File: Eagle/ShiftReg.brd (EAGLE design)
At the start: 100 x 80 mm, 206 parts, among them Q10 310mA/60V/1.6Ω, Q100 310mA/60V/1.6Ω, Q101 310mA/60V/1.6Ω, Q102 310mA/60V/1.6Ω, Q103 310mA/60V/1.6Ω, Q104 310mA/60V/1.6Ω, Q105 310mA/60V/1.6Ω, Q106 310mA/60V/1.6Ω, Q107 310mA/60V/1.6Ω, Q108 310mA/60V/1.6Ω, Q109 310mA/60V/1.6Ω, Q11 310mA/60V/1.6Ω, Q110 310mA/60V/1.6Ω, Q111 310mA/60V/1.6Ω, Q112 310mA/60V/1.6Ω, Q113 310mA/60V/1.6Ω, Q114 310mA/60V/1.6Ω, Q115 310mA/60V/1.6Ω, Q116 310mA/60V/1.6Ω, Q117 310mA/60V/1.6Ω, Q118 310mA/60V/1.6Ω, Q119 310mA/60V/1.6Ω, Q12 310mA/60V/1.6Ω, Q120 310mA/60V/1.6Ω, Q121 310mA/60V/1.6Ω, Q122 310mA/60V/1.6Ω, Q123 310mA/60V/1.6Ω, Q124 310mA/60V/1.6Ω, Q125 310mA/60V/1.6Ω, Q126 310mA/60V/1.6Ω, Q127 310mA/60V/1.6Ω, Q128 310mA/60V/1.6Ω, Q129 310mA/60V/1.6Ω, Q13 310mA/60V/1.6Ω, Q130 310mA/60V/1.6Ω, Q131 310mA/60V/1.6Ω, Q132 310mA/60V/1.6Ω, Q133 310mA/60V/1.6Ω, Q134 310mA/60V/1.6Ω, Q135 310mA/60V/1.6Ω, Q136 310mA/60V/1.6Ω, Q137 310mA/60V/1.6Ω, Q138 310mA/60V/1.6Ω, Q139 310mA/60V/1.6Ω, Q14 310mA/60V/1.6Ω, Q140 310mA/60V/1.6Ω, Q141 310mA/60V/1.6Ω, Q142 310mA/60V/1.6Ω, Q143 310mA/60V/1.6Ω, Q144 310mA/60V/1.6Ω, Q145 310mA/60V/1.6Ω, Q146 310mA/60V/1.6Ω, Q147 310mA/60V/1.6Ω, Q148 310mA/60V/1.6Ω, Q149 310mA/60V/1.6Ω, Q15 310mA/60V/1.6Ω, Q150 310mA/60V/1.6Ω, Q151 310mA/60V/1.6Ω, Q152 310mA/60V/1.6Ω, Q153 310mA/60V/1.6Ω, Q154 310mA/60V/1.6Ω, Q155 310mA/60V/1.6Ω, Q156 310mA/60V/1.6Ω, Q157 310mA/60V/1.6Ω, Q158 310mA/60V/1.6Ω, Q159 310mA/60V/1.6Ω, Q16 310mA/60V/1.6Ω, Q160 310mA/60V/1.6Ω, Q161 310mA/60V/1.6Ω, Q162 310mA/60V/1.6Ω, Q163 310mA/60V/1.6Ω, Q164 310mA/60V/1.6Ω, Q165 310mA/60V/1.6Ω, Q25 310mA/60V/1.6Ω, Q26 310mA/60V/1.6Ω, Q27 310mA/60V/1.6Ω, Q28 310mA/60V/1.6Ω, Q29 310mA/60V/1.6Ω, Q30 310mA/60V/1.6Ω, Q31 310mA/60V/1.6Ω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

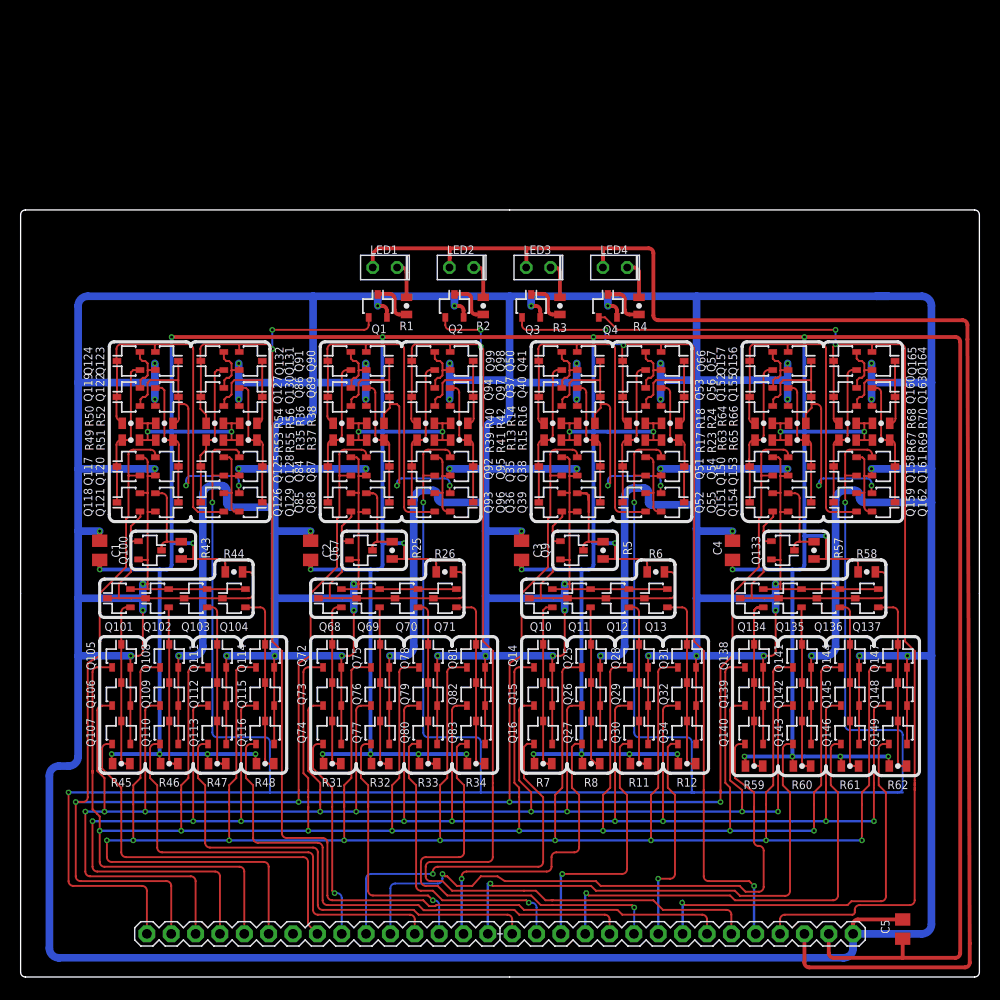
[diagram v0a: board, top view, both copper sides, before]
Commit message: Updated boards with pcb template
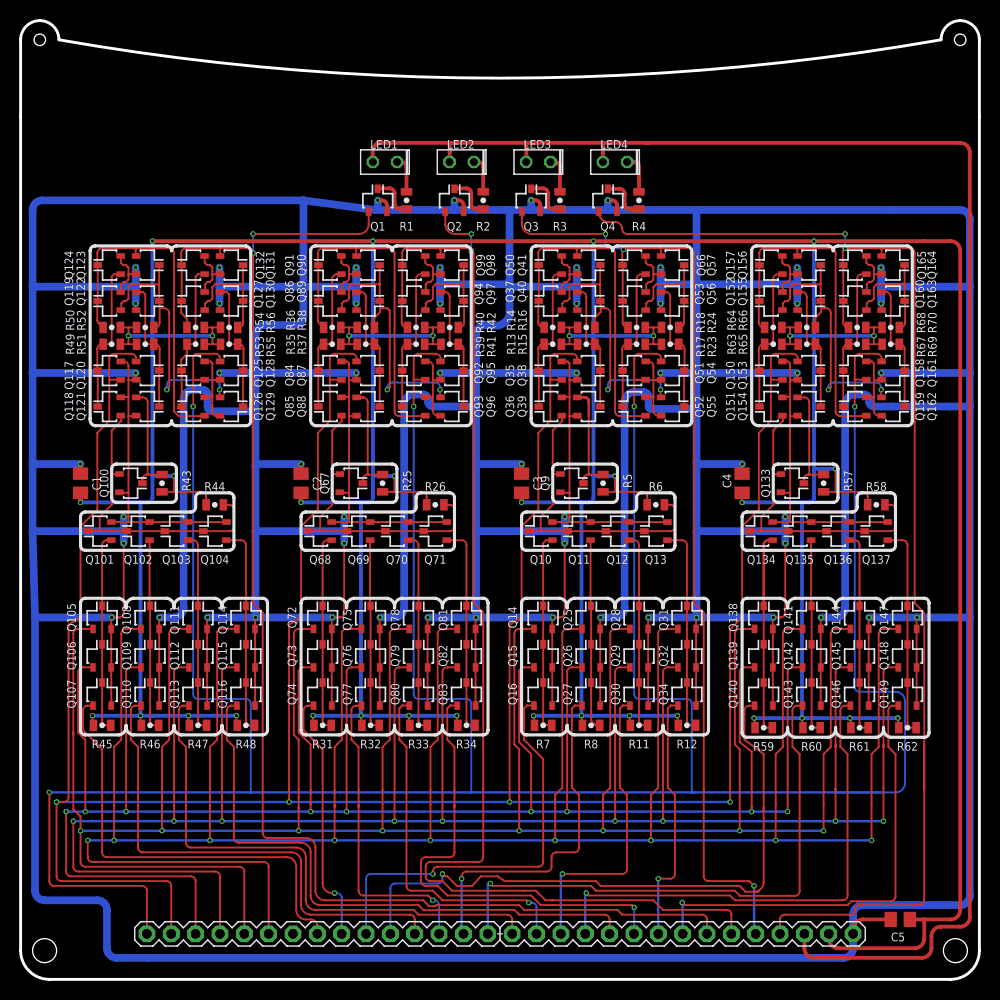
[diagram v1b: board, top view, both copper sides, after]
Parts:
- moved LED1 11.0 mm to (38.0, 85.0)
- moved LED2 11.0 mm to (46.0, 85.0)
- moved LED3 11.0 mm to (54.0, 85.0)
- moved LED4 11.0 mm to (62.0, 85.0)
- moved Q1 11.0 mm to (37.2, 81.0)
- moved Q2 11.0 mm to (45.2, 81.0)
- moved Q3 11.0 mm to (53.2, 81.0)
- moved Q4 11.0 mm to (61.2, 81.0)
- moved R1 11.0 mm to (40.2, 81.0)
- moved R2 11.0 mm to (48.2, 81.0)
- moved R3 11.0 mm to (56.2, 81.0)
- moved R4 11.0 mm to (64.5, 81.0)
- moved Q117 10.2 mm to (9.25, 63.2)
- moved Q118 10.2 mm to (9.25, 59.5)
- moved Q119 10.2 mm to (9.25, 70.5)
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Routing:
- net GND: track 1200.5 -> 1333.8 mm
- net /CLK: track 263.0 -> 308.0 mm
- net CLK: track 295.2 -> 339.8 mm
- net OP2: track 252.9 -> 289.9 mm
- net OP1: track 196.8 -> 233.8 mm
- net /OP2: track 266.5 -> 303.5 mm
- net /OP1: track 213.3 -> 250.3 mm
- net VCC: track 563.9 -> 595.9 mm
- net OUT3: track 118.6 -> 136.0 mm
- net OUT0: track 133.7 -> 147.8 mm
- net OUT2: track 96.5 -> 107.2 mm
- net OUT1: track 121.0 -> 129.7 mm
- net LED+: track 164.0 -> 172.0 mm
- net PREV3A': track 22.6 -> 28.6 mm
- net NEXT0: track 46.6 -> 52.0 mm
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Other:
- board size 100 x 80 mm -> 100 x 100 mm
- board text added: "Universal shiftregister rev1"
- board text removed: "Universal Shiftregister rev 1"
